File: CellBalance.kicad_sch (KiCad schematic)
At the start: 9 parts

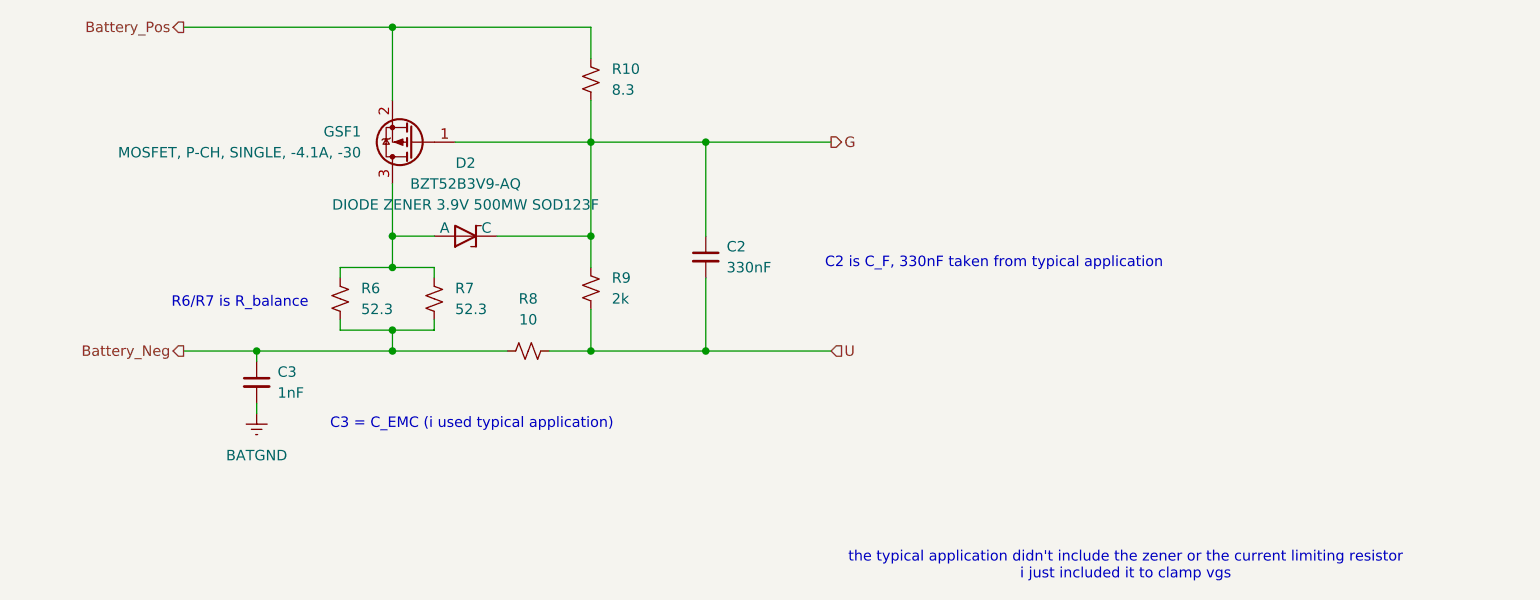
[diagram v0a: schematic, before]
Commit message: finished schematic
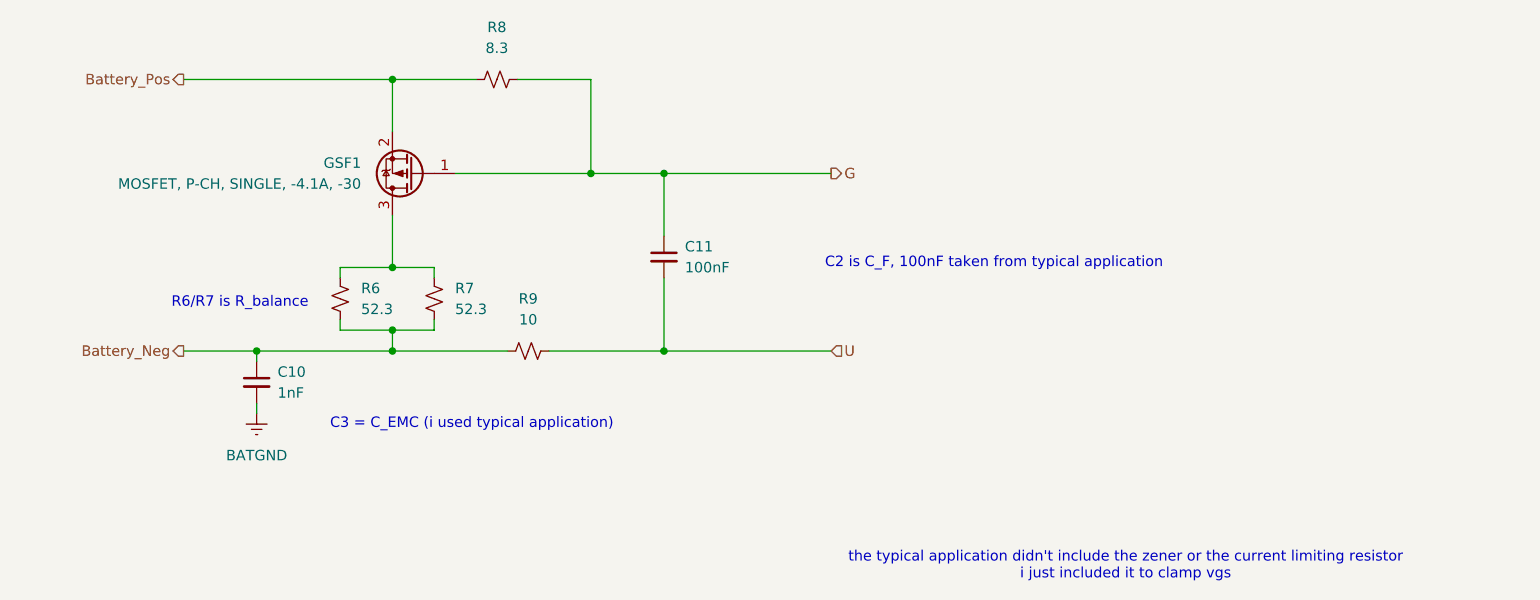
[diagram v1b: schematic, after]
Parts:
- removed D2: BZT52B3V9-AQ, footprints:P35_SOD-123F, symbol symbols:Diode
- removed R10: 8.3, symbol Device:R_Small_US
- removed R9: 2k, symbol Device:R_Small_US
- added R8: 8.3, symbol Device:R_Small_US
- C11: renamed from C2; value 330nF -> 100nF
- renumbered C3 to C10, R8 to R9
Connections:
- net Battery_Pos: now also R8.2
- net G: now also R8.1
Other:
- note added: "C2 is C_F, 100nF taken from typical application"
- note removed: "C2 is C_F, 330nF taken from typical application"
- moved on the sheet: C11, GSF1
